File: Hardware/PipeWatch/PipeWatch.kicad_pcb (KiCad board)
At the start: 2 copper layers, 100.2 x 100.1 mm, 20 parts, among them J1 WJ126V-5.0-2P, J2 Conn_01x04_Pin, J3 UART, J4 JTAG, U1 IRM-10-5_C20618064, U3 ESP32-S3-WROOM-1-N16R8, U5 XIAO-ESP32-S3-DIP

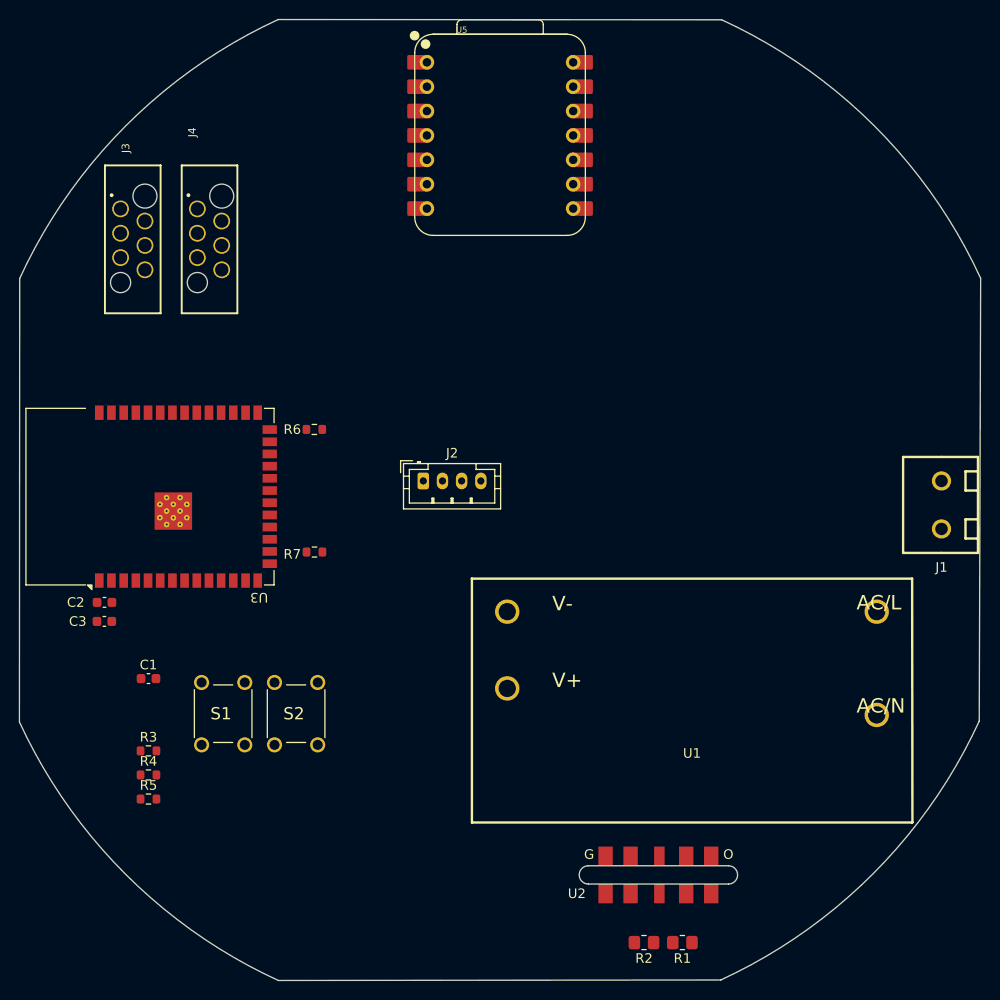
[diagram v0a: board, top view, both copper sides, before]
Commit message: tweeked the Layout
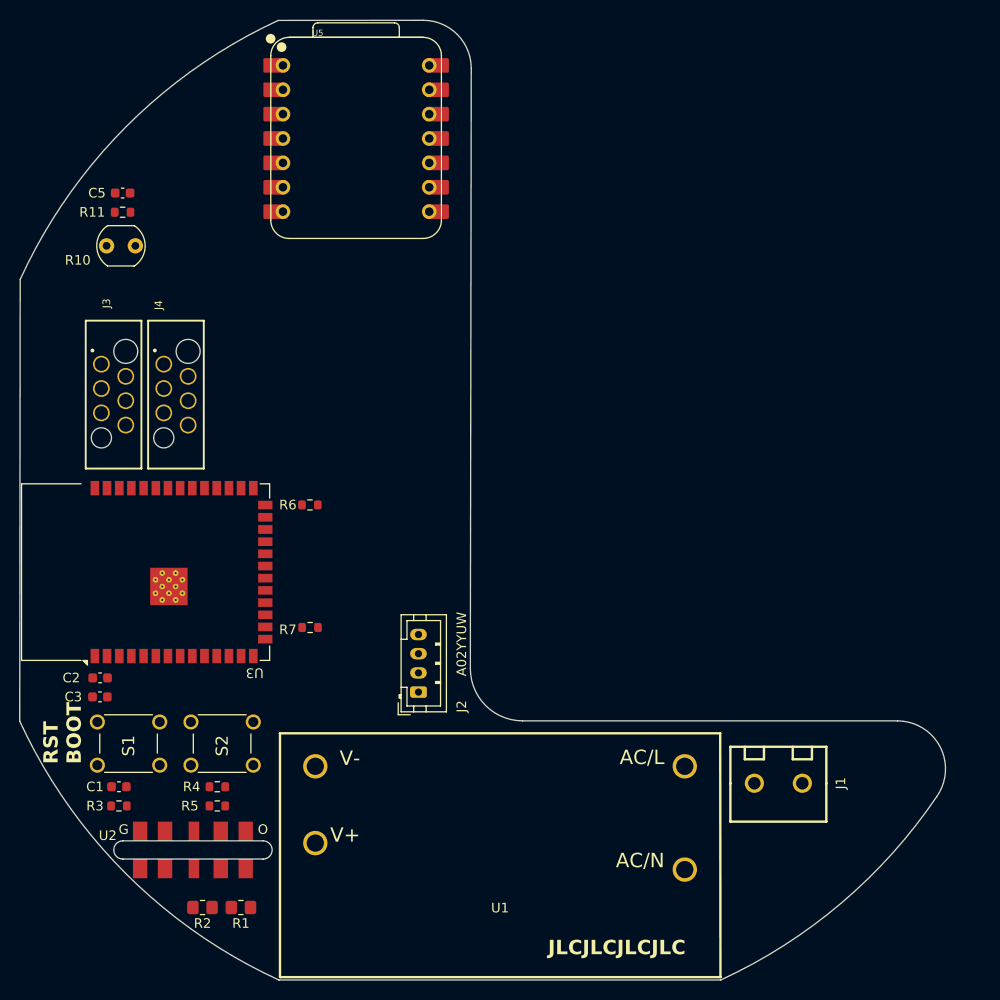
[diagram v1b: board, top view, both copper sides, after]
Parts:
- added C5: 10n, Capacitor_SMD:C_0603_1608Metric, F.Cu at (100.7, 68.0)
- added R10: R_Photo, OptoDevice:R_LDR_5.0x4.1mm_P3mm_Vertical, F.Cu at (102.0, 73.5)
- added R11: 10M, Resistor_SMD:R_0603_1608Metric, F.Cu at (100.7, 70.0)
- J2: value Conn_01x04_Pin -> A02YYUW
- moved U2 48.6 mm to (99.8, 137.4)
- moved R1 46.1 mm to (113.0, 142.4)
- moved R2 46.1 mm to (109.0, 142.4)
- moved J1 33.6 mm to (169.0, 129.5), turned to -90 degrees
- moved U1 25.7 mm to (140.0, 133.1)
- moved J2 22.0 mm to (131.5, 120.0), turned to 90 degrees
- moved J4 16.6 mm to (106.2, 89.0)
- moved J3 16.3 mm to (99.7, 89.0)
- moved U5 15.0 mm to (125.0, 62.3)
- moved S1 13.9 mm to (98.0, 127.6), turned to 90 degrees
- moved S2 12.3 mm to (107.8, 127.6), turned to 90 degrees
- moved C1 11.7 mm to (100.3, 129.9)
- moved R7 7.88 mm to (120.2, 113.3)
- moved C2 7.88 mm to (98.3, 118.5)
- moved C3 7.88 mm to (98.3, 120.5)
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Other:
- board size 100.2 x 100.1 mm -> 96.5 x 100 mm
- board text added: "JLCJLCJLCJLC"
- board text added: "RST BOOT"
